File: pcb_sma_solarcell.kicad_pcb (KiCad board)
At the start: 2 copper layers, 35.5 x 120.2 mm, 5 parts, among them J1 CON-SMA-EDGE-S, J2 CON-SMA-EDGE-S, J3 CON-SMA-EDGE-S, J4 CON-SMA-EDGE-S

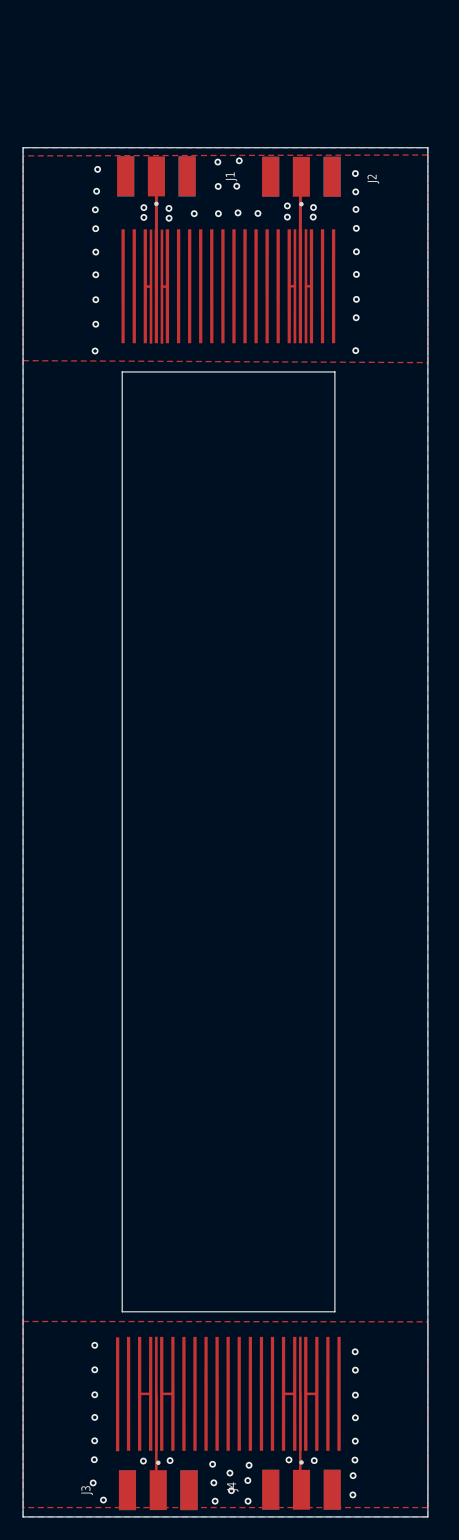
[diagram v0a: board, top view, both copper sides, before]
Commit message: Describe what changed
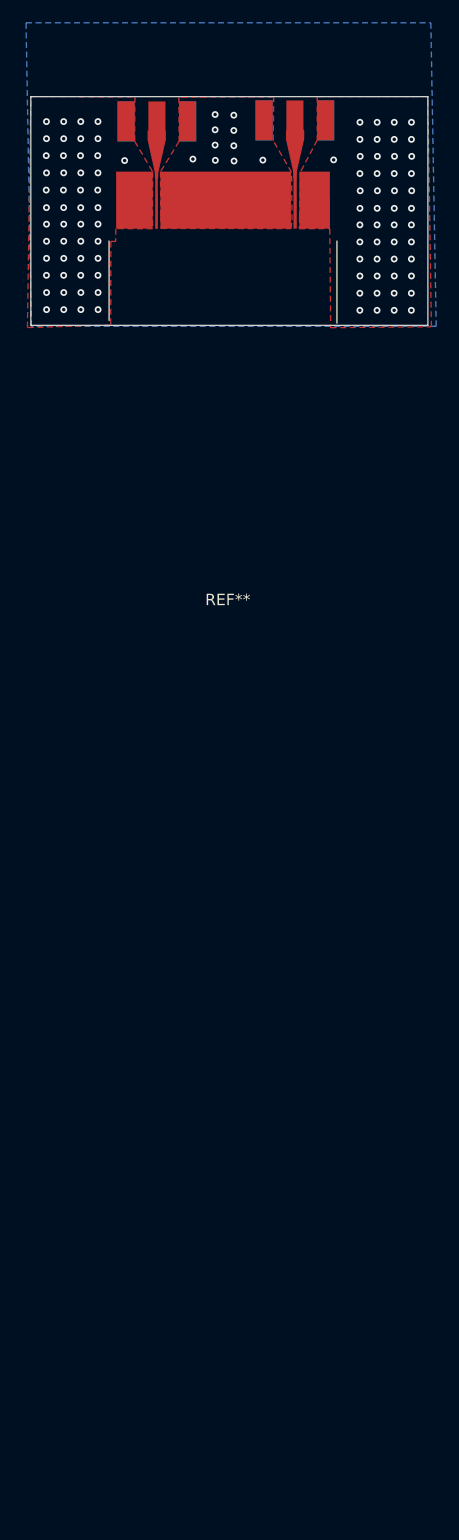
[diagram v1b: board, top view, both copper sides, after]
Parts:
- removed J3, J4: CON-SMA-EDGE-S, Library:RFSOLUTIONS_CON-SMA-EDGE-S
- removed U1: ~, Library:sma_topandbot
- added REF**: footprint_sma_oneside, Library:footprint_sma_oneside, F.Cu at (73.6, 67.5)
- moved J2 4.98 mm to (79.5, 24.9)
- moved J1 4.83 mm to (67.4, 25.0)
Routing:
- net /V2: track 9.64 -> 0.00 mm
- net /V1: track 9.64 -> 0.00 mm
- net /GND: track 10.3 -> 0.75 mm, vias 62 -> 108
- net /V3: track 8.53 -> 0.00 mm
- net /V4: track 8.47 -> 0.00 mm
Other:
- board size 35.5 x 120.2 mm -> 34.8 x 20.1 mm
- board text added: "Nom: Catherine Bourget Version: 03/02/2026"
